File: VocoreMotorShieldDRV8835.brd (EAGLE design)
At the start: 100 x 80 mm, 9 parts

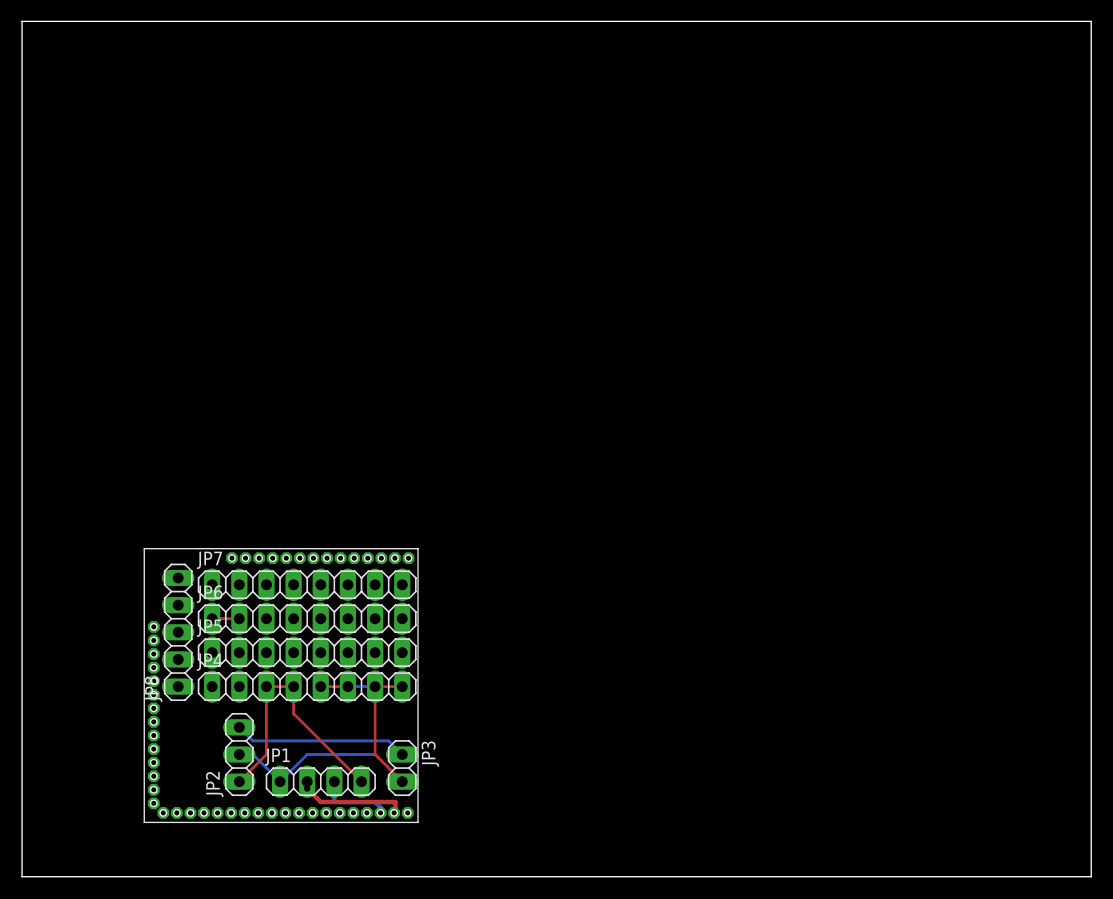
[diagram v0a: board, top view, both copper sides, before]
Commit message: Version 0.2
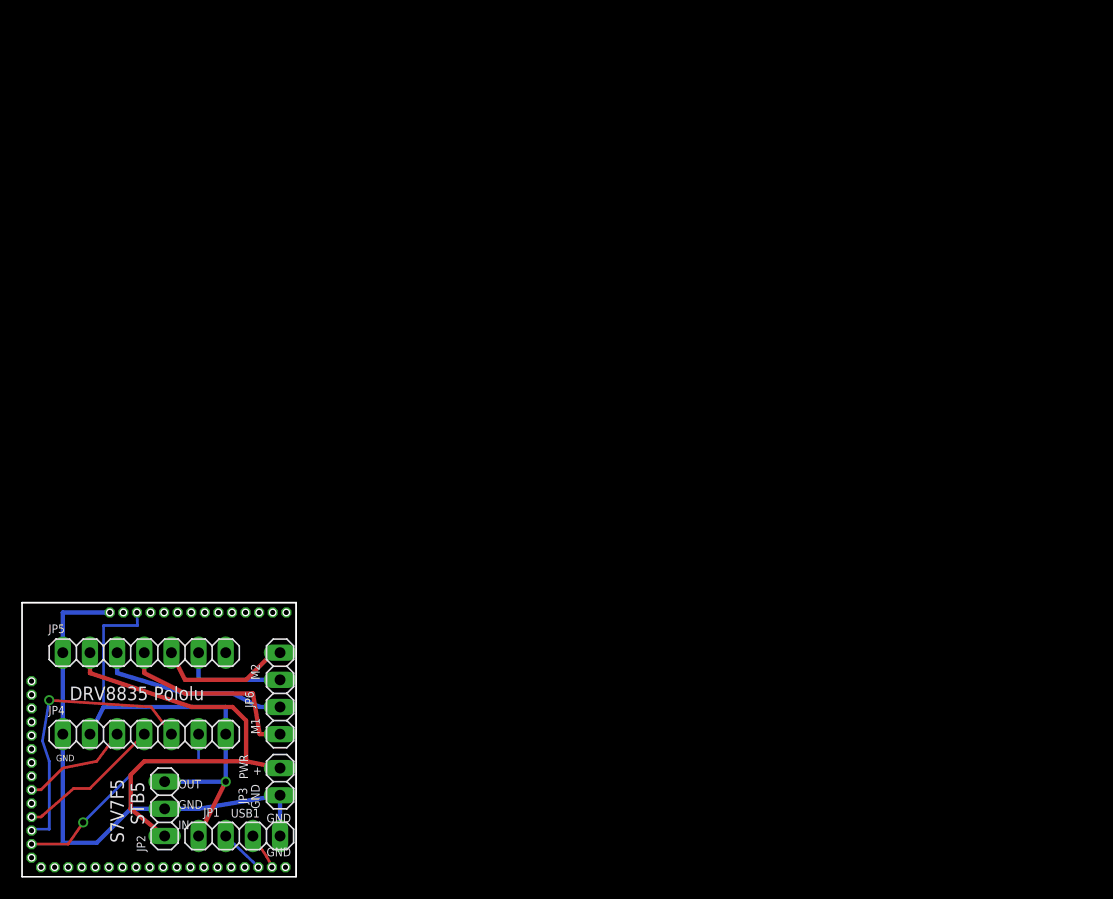
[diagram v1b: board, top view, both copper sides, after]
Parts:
- removed JP7: (no value), pinhead:1X08
- removed JP8: (no value), pinhead:1X05
- removed U$1: VOCORE_SHIELD, Vocore:VOCORE_DOC_CUSTOM
- added U1: VOCORE_SHIELD, Vocore:VOCORE_DOC_CUSTOM
- JP4, JP5: device pinhead:1X08 -> pinhead:1X07
- JP6: device pinhead:1X08 -> pinhead:1X04
- moved JP4 15.9 mm to (11.4, 13.3)
- moved JP5 15.2 mm to (11.4, 21.0)
- moved JP3 11.5 mm to (24.1, 8.89)
- moved JP1 9.16 mm to (20.3, 3.81), turned to 180 degrees
- moved JP2 8.64 mm to (13.3, 6.35), turned to 270 degrees
- moved JP6 7.43 mm to (24.1, 17.1), turned to 90 degrees
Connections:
- removed net N$12: JP5.5, U$1.G#24/LED2
- removed net N$15: JP5.8, U$1.G#27/SPI_CS1
- removed net N$16: JP6.8, U$1.G#14/PCM_TDX
- removed net N$17: JP6.7, U$1.G#13/PCM_DRX
- removed net N$18: JP6.6, U$1.G#12/PCM_CLK
- removed net N$19: JP6.5, U$1.G#11/PCM_FS
- removed net N$20: JP6.4, U$1.G#10/I2S_SDI/RXD
- removed net N$21: JP6.3, U$1.G#09/I2S_SDO
- removed net N$22: JP6.1, JP6.2, U$1.G#08/I2S_WS/TXD
- removed net N$23: JP7.1, U$1.RESET
- removed net N$24: JP7.2, U$1.G#00
- removed net N$25: JP7.3, U$1.G#01/I2C_CLK
- removed net N$26: JP7.4, U$1.G#02/I2C_SD
- removed net N$27: JP7.5, U$1.G#03/SPI_CS0
- removed net N$28: JP7.6, U$1.G#04/SPI_CLK
- removed net N$29: JP7.7, U$1.G#05/SPI_MOSI
- removed net N$30: JP7.8, U$1.G#06/SPI_MISO
- removed net N$31: JP8.2, U$1.G#20/JTAG_TCLK
- removed net N$32: U$1.G#19/JTAG_TMS
- removed net N$33: JP8.4, U$1.G#18/JTAG_TDI
- removed net N$34: JP8.1, U$1.G#21/JTAG_TRST
- removed net N$35: JP8.5, U$1.G#17/JTAG_TDO
- net N$1: now also JP4.1, JP5.1, U1.GND2; no longer JP4.5, JP4.6, JP4.7, JP4.8, U$1.GND, U$1.GND1, U$1.GND2, U$1.GND3
- net N$10: now also JP5.4, JP6.1; no longer JP5.3, U$1.G#22/LED0
- net N$11: now also JP5.3, JP6.2; no longer JP5.4, U$1.G#23/LED1
- net N$13: now also JP5.5, JP6.4; no longer JP5.6, U$1.G#25/LED3
- net N$14: now also JP5.6, JP6.3; no longer JP5.7, U$1.G#26/LED4
- net N$2: now also JP5.2
- net N$3: now also JP4.2, JP4.7, U1.+6.0VIN1; no longer JP4.3, JP4.4, U$1.+6.0VIN, U$1.+6.0VIN1
- net N$4: now also JP4.3, U1.G#23/LED1; no longer JP4.1, U$1.+1.8V
- net N$5: now also U1.USB-; no longer U$1.USB-
- net N$6: now also U1.USB+; no longer U$1.USB+
- net N$7: now also JP4.4, U1.G#24/LED2; no longer JP4.2, U$1.+3.2V~+3.5V
- net N$8: now also JP4.5, U1.G#25/LED3; no longer JP5.1, U$1.G#15/TXD2
- net N$9: now also JP4.6, U1.G#26/LED4; no longer JP5.2, U$1.G#16/RXD2
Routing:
- net N$2: track 16.3 -> 43.2 mm
- net N$8: track 0.00 -> 26.6 mm, vias 0 -> 1
- net N$9: track 0.00 -> 21.6 mm, vias 0 -> 1
- net N$3: track 24.0 -> 44.7 mm, vias 0 -> 1
- net N$10: track 0.00 -> 18.3 mm
- net N$11: track 0.00 -> 17.7 mm
- net N$1: track 36.0 -> 51.5 mm, vias 0 -> 1
- net N$7: track 0.00 -> 13.6 mm
- net N$13: track 0.00 -> 12.8 mm
- net N$4: track 0.00 -> 10.2 mm
- net N$14: track 0.00 -> 10.2 mm
- net N$6: track 10.5 -> 3.78 mm, vias 1 -> 0
- net N$5: track 6.94 -> 4.22 mm
- net N$22: track 2.54 -> 0.00 mm
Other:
- board size 100 x 80 mm -> 25.7 x 25.7 mm
- board text added: "+"
- board text added: "DRV8835 Pololu"
- board text added: "GND"
- board text added: "IN"
- board text added: "M1"
- board text added: "M2"
- board text added: "OUT"
- board text added: "S7V7F5"
